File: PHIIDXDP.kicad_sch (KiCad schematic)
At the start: 45 parts, among them J1 USB_C_Receptacle_USB2.0_16P, J10 2P BT 2, J11 2P BT 3, J12 2P BT 4, J13 2P BT 5, J14 2P BT 6, J15 2P BT 7, J16 1P START, J17 EFFECT, J18 VEFX, J19 2P START, J2 1P BT 1, J20 P1 TT analog, J21 P2 TT analog, J22 LED P1 TT, J23 LED P2 TT, J24 LED P1 Buttons, J25 LED P2 Buttons, J26 LED CENTER, J28 P1 TT Encoder, J29 P2 TT Encoder, J3 1P BT 3, J4 1P BT 5, J5 1P BT 7, J6 1P BT 2, J7 1P BT 4, J8 1P BT 6, J9 2P BT 1, SW1 SW_Push, U1 AT90USB647-A, Y1 16MHz

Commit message: symbol VOMIT
updated footprints and started PCB work lol
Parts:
- SW1: footprint (none) -> Button_Switch_SMD:SW_SPST_SKQG_WithStem
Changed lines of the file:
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@@
 			)
 		)
-		(property "Footprint" ""
+		(property "Footprint" "Button_Switch_SMD:SW_SPST_SKQG_WithStem"
 			(at 102.87 29.21 0)
 			(effects

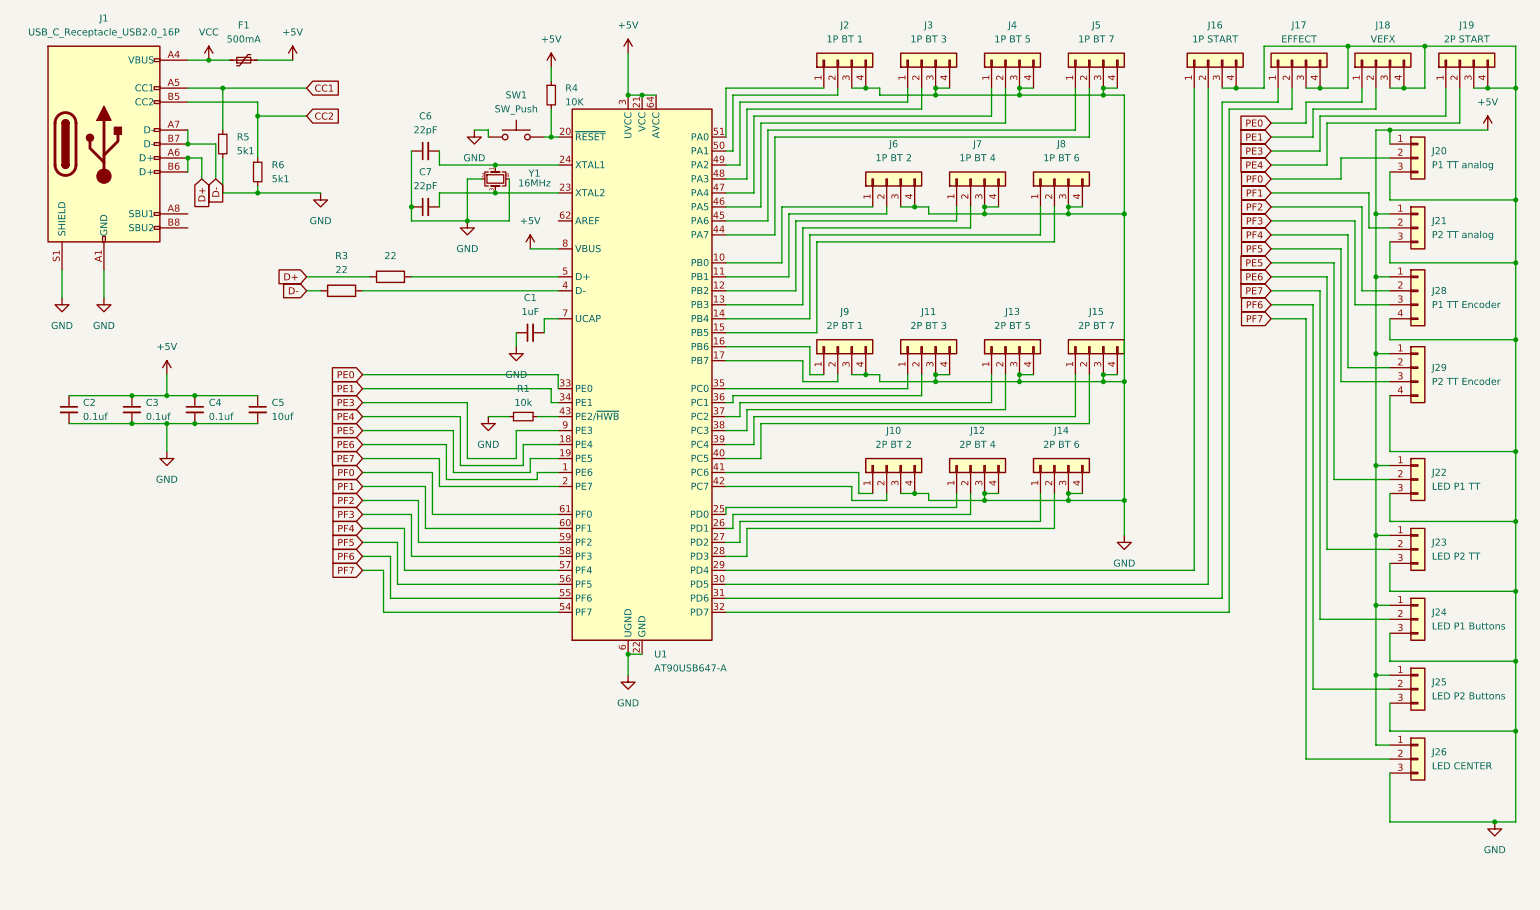
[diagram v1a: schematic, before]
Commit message: Reworking stuffs
reworking schematic whilst tracing the PCB at the same time how fun!!!!
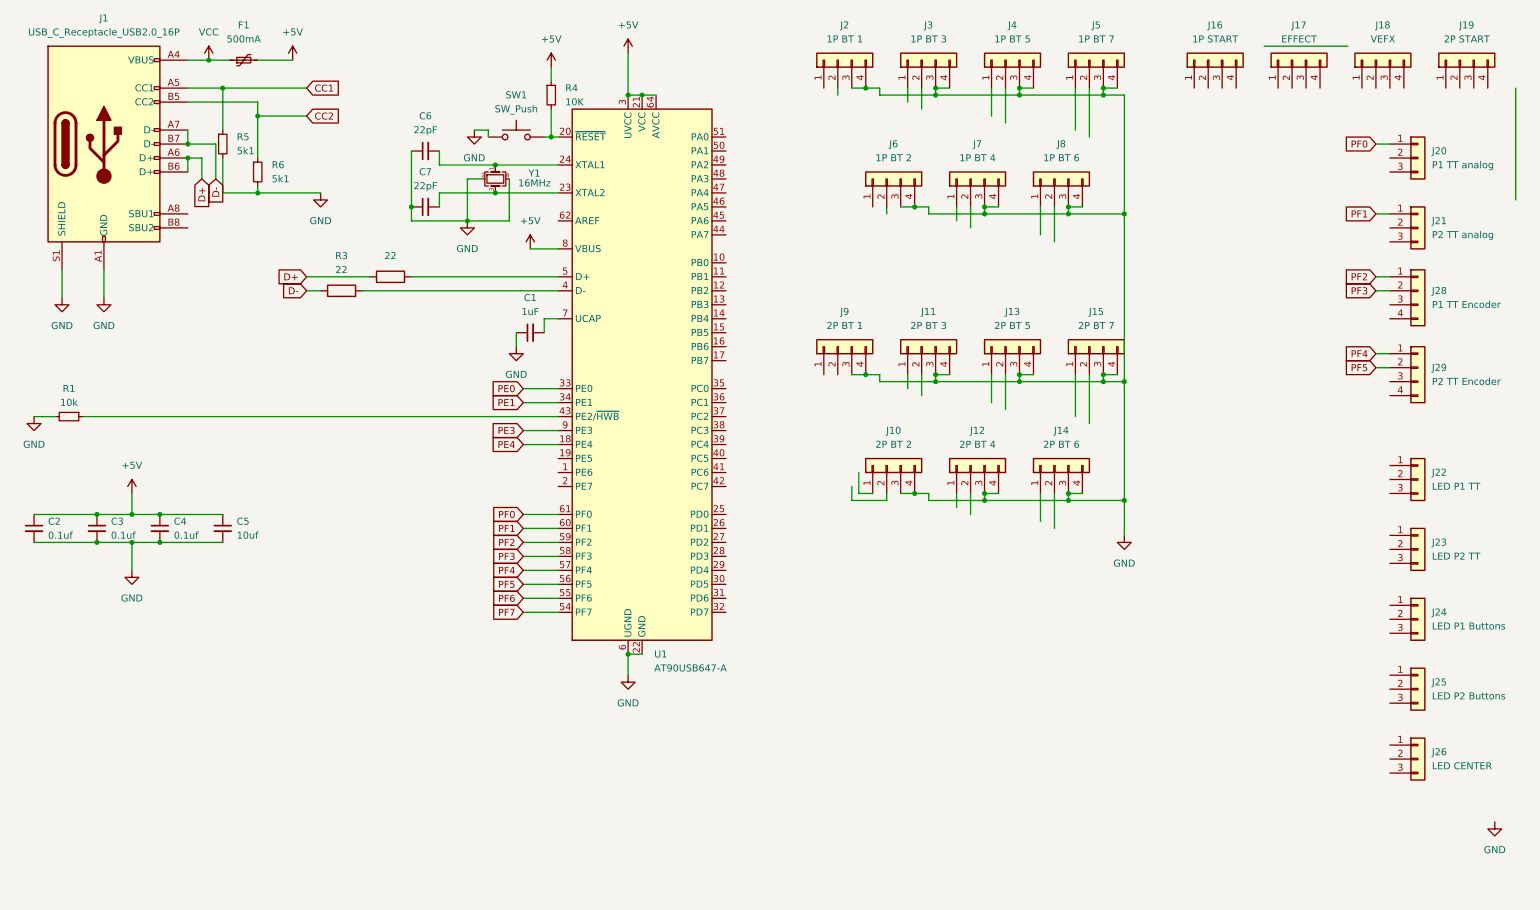
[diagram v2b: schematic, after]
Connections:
- net +5V: no longer J20.1 (Pin_1), J21.1 (Pin_1), J22.1 (Pin_1), J23.1 (Pin_1), J24.1 (Pin_1), J25.1 (Pin_1), J26.1 (Pin_1), J28.1 (Pin_1), J29.1 (Pin_1)
- net GND: no longer J16.3 (Pin_3), J16.4 (Pin_4), J17.3 (Pin_3), J17.4 (Pin_4), J18.3 (Pin_3), J18.4 (Pin_4), J19.3 (Pin_3), J19.4 (Pin_4), J20.3 (Pin_3), J21.3 (Pin_3), J22.3 (Pin_3), J23.3 (Pin_3), J24.3 (Pin_3), J25.3 (Pin_3), J26.3 (Pin_3), J28.4 (Pin_4), J29.4 (Pin_4)
- net PE0: no longer J18.1 (Pin_1)
- net PE1: no longer J18.2 (Pin_2)
- net PE3: no longer J19.1 (Pin_1)
- net PE4: no longer J19.2 (Pin_2)
- net PF0: now also J20.1 (Pin_1); no longer J20.2 (Pin_2)
- net PF1: now also J21.1 (Pin_1); no longer J21.2 (Pin_2)
- net PF2: now also J28.1 (Pin_1); no longer J28.2 (Pin_2)
- net PF3: now also J28.2 (Pin_2); no longer J28.3 (Pin_3)
- net PF4: now also J29.1 (Pin_1); no longer J29.2 (Pin_2)
- net PF5: now also J29.2 (Pin_2); no longer J29.3 (Pin_3)
- net PF6: no longer J25.2 (Pin_2)
- net PF7: no longer J26.2 (Pin_2)
- net at J10.1 (Pin_1): no longer U1.41 (PC6)
- net at J10.2 (Pin_2): no longer U1.42 (PC7)
- net at J16.1 (Pin_1): no longer U1.29 (PD4)
- net at J16.2 (Pin_2): no longer U1.30 (PD5)
- net at J8.1 (Pin_1): no longer U1.14 (PB4)
- net at J8.2 (Pin_2): no longer U1.15 (PB5)
- net at J2.1 (Pin_1): no longer U1.51 (PA0)
- net at J2.2 (Pin_2): no longer U1.50 (PA1)
- net at J6.1 (Pin_1): no longer U1.10 (PB0)
- net at J6.2 (Pin_2): no longer U1.11 (PB1)
- net at J17.1 (Pin_1): no longer U1.31 (PD6)
- net at J17.2 (Pin_2): no longer U1.32 (PD7)
- net at J13.1 (Pin_1): no longer U1.37 (PC2)
- net at J13.2 (Pin_2): no longer U1.38 (PC3)
- net at J5.1 (Pin_1): no longer U1.45 (PA6)
- net at J5.2 (Pin_2): no longer U1.44 (PA7)
- net at U1.12 (PB2): no longer J7.1 (Pin_1)
- net at U1.13 (PB3): no longer J7.2 (Pin_2)
- net at U1.16 (PB6): no longer J9.1 (Pin_1)
- net at U1.17 (PB7): no longer J9.2 (Pin_2)
- net at U1.25 (PD0): no longer J12.1 (Pin_1)
- net at U1.26 (PD1): no longer J12.2 (Pin_2)
- net at U1.27 (PD2): no longer J14.1 (Pin_1)
- net at U1.28 (PD3): no longer J14.2 (Pin_2)
- net at U1.35 (PC0): no longer J11.1 (Pin_1)
- net at U1.36 (PC1): no longer J11.2 (Pin_2)
- net at U1.39 (PC4): no longer J15.1 (Pin_1)
- net at U1.40 (PC5): no longer J15.2 (Pin_2)
- net at U1.46 (PA5): no longer J4.2 (Pin_2)
- net at U1.47 (PA4): no longer J4.1 (Pin_1)
- net at U1.48 (PA3): no longer J3.2 (Pin_2)
- net at U1.49 (PA2): no longer J3.1 (Pin_1)
- net PE5: no longer names the net of U1.19 (PE5)
- net PE5: no longer J22.2 (Pin_2)
- net PE6: no longer names the net of U1.1 (PE6)
- net PE6: no longer J23.2 (Pin_2)
- net PE7: no longer names the net of J24.2 (Pin_2)
- net PE7: no longer U1.2 (PE7)
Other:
- moved on the sheet: C2, C3, C4, C5, R1

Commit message: I forgot to commit this oopsiedaisies
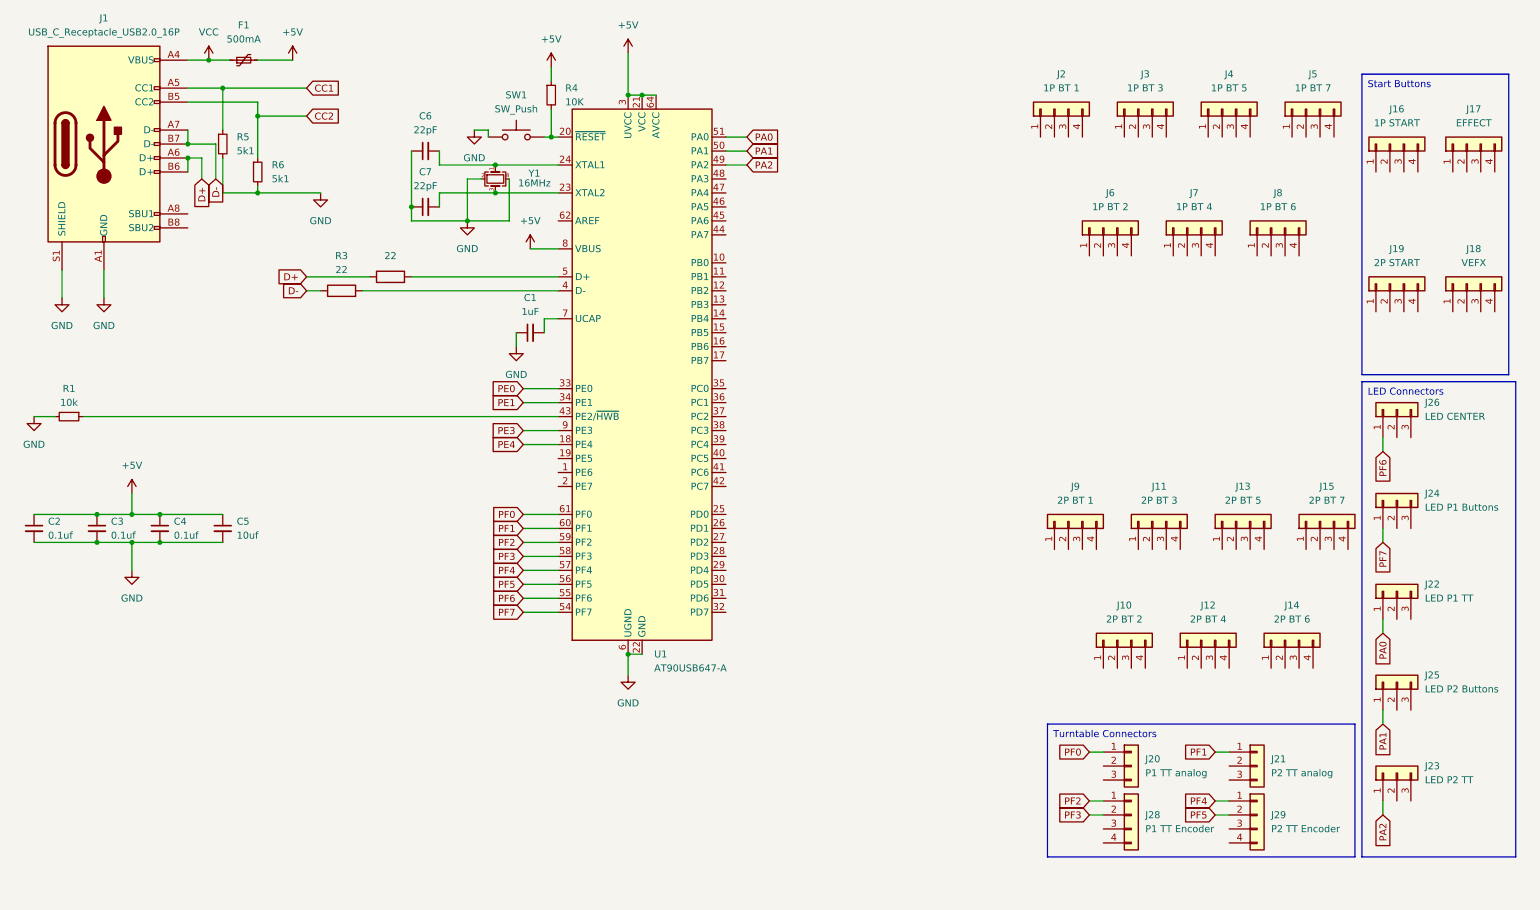
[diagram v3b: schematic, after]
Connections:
- net GND: no longer J10.3 (Pin_3), J10.4 (Pin_4), J11.3 (Pin_3), J11.4 (Pin_4), J12.3 (Pin_3), J12.4 (Pin_4), J13.3 (Pin_3), J13.4 (Pin_4), J14.3 (Pin_3), J14.4 (Pin_4), J15.3 (Pin_3), J15.4 (Pin_4), J2.3 (Pin_3), J2.4 (Pin_4), J3.3 (Pin_3), J3.4 (Pin_4), J4.3 (Pin_3), J4.4 (Pin_4), J5.3 (Pin_3), J5.4 (Pin_4), J6.3 (Pin_3), J6.4 (Pin_4), J7.3 (Pin_3), J7.4 (Pin_4), J8.3 (Pin_3), J8.4 (Pin_4), J9.3 (Pin_3), J9.4 (Pin_4)
- net PF6: now also J26.1 (Pin_1)
- net PF7: now also J24.1 (Pin_1)
- net PA2: now reaches U1.49 (PA2)
- net PA2: now also J23.1 (Pin_1)
- net PA1: now reaches U1.50 (PA1)
- net PA1: now also J25.1 (Pin_1)
- net PA0: now reaches U1.51 (PA0)
- net PA0: now also J22.1 (Pin_1)
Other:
- moved on the sheet: J10, J11, J12, J13, J14, J15, J16, J17, J18, J19, J2, J20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

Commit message: AAAAAAAA
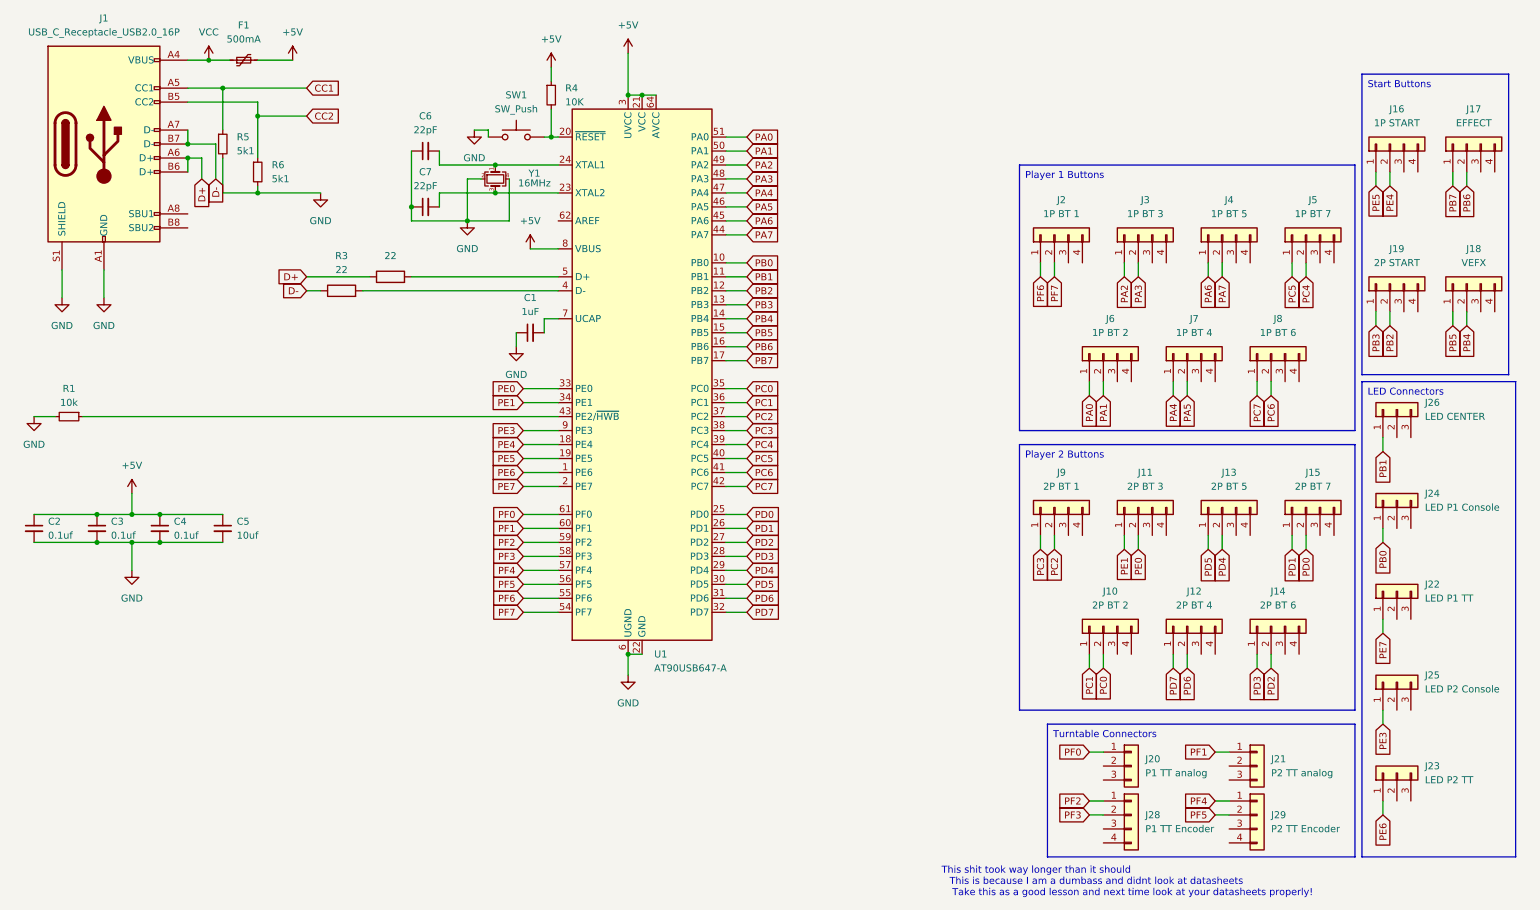
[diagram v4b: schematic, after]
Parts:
- J24: value LED P1 Buttons -> LED P1 Console
- J25: value LED P2 Buttons -> LED P2 Console
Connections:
- net PA0: now also J6.1 (Pin_1); no longer J22.1 (Pin_1)
- net PA1: now also J6.2 (Pin_2); no longer J25.1 (Pin_1)
- net PA2: now also J3.1 (Pin_1); no longer J23.1 (Pin_1)
- net PE0: now also J11.2 (Pin_2)
- net PE1: now also J11.1 (Pin_1)
- net PE3: now also J25.1 (Pin_1)
- net PE4: now also J16.2 (Pin_2)
- net PF6: now also J2.1 (Pin_1); no longer J26.1 (Pin_1)
- net PF7: now also J2.2 (Pin_2); no longer J24.1 (Pin_1)
- net PC1: now reaches J10.1 (Pin_1)
- net PC1: now also U1.36 (PC1)
- net PC0: now reaches J10.2 (Pin_2)
- net PC0: now also U1.35 (PC0)
- net PE5: now reaches J16.1 (Pin_1)
- net PE5: now also U1.19 (PE5)
- net PC7: now reaches J8.1 (Pin_1)
- net PC7: now also U1.42 (PC7)
- net PC6: now reaches J8.2 (Pin_2)
- net PC6: now also U1.41 (PC6)
- net PB3: now reaches J19.1 (Pin_1)
- net PB3: now also U1.13 (PB3)
- net PB2: now reaches J19.2 (Pin_2)
- net PB2: now also U1.12 (PB2)
- net PB7: now reaches J17.1 (Pin_1)
- net PB7: now also U1.17 (PB7)
- net PB6: now reaches J17.2 (Pin_2)
- net PB6: now also U1.16 (PB6)
- net PD5: now reaches J13.1 (Pin_1)
- net PD5: now also U1.30 (PD5)
- net PD4: now reaches J13.2 (Pin_2)
- net PD4: now also U1.29 (PD4)
- net PC5: now reaches J5.1 (Pin_1)
- net PC5: now also U1.40 (PC5)
- net PC4: now reaches J5.2 (Pin_2)
- net PC4: now also U1.39 (PC4)
- net PE6: now reaches U1.1 (PE6)
- net PE6: now also J23.1 (Pin_1)
- net PB0: now reaches U1.10 (PB0)
- net PB0: now also J24.1 (Pin_1)
- net PB1: now reaches U1.11 (PB1)
- net PB1: now also J26.1 (Pin_1)
- net PB4: now reaches U1.14 (PB4)
- net PB4: now also J18.2 (Pin_2)
- net PB5: now reaches U1.15 (PB5)
- net PB5: now also J18.1 (Pin_1)
- net PE7: now reaches U1.2 (PE7)
- net PE7: now also J22.1 (Pin_1)
- net PD0: now reaches U1.25 (PD0)
- net PD0: now also J15.2 (Pin_2)
- net PD1: now reaches U1.26 (PD1)
- net PD1: now also J15.1 (Pin_1)
- net PD2: now reaches U1.27 (PD2)
- net PD2: now also J14.2 (Pin_2)
- net PD3: now reaches U1.28 (PD3)
- net PD3: now also J14.1 (Pin_1)
- net PD6: now reaches U1.31 (PD6)
- net PD6: now also J12.2 (Pin_2)
- net PD7: now reaches U1.32 (PD7)
- net PD7: now also J12.1 (Pin_1)
- net PC2: now reaches U1.37 (PC2)
- net PC2: now also J9.2 (Pin_2)
- net PC3: now reaches U1.38 (PC3)
- net PC3: now also J9.1 (Pin_1)
- net PA7: now reaches U1.44 (PA7)
- net PA7: now also J4.2 (Pin_2)
- net PA6: now reaches U1.45 (PA6)
- net PA6: now also J4.1 (Pin_1)
- net PA5: now reaches U1.46 (PA5)
- net PA5: now also J7.2 (Pin_2)
- net PA4: now reaches U1.47 (PA4)
- net PA4: now also J7.1 (Pin_1)
- net PA3: now reaches U1.48 (PA3)
- net PA3: now also J3.2 (Pin_2)
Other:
- note added: "Take this as a good lesson and next time look at your datasheets properly!"
- note added: "This is because I am a dumbass and didnt look at datasheets"
- note added: "This shit took way longer than it should"
- moved on the sheet: J10, J11, J12, J13, J14, J15, J2, J3, J4, J5, J6, J7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
